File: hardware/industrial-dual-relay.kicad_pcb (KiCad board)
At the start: 2 copper layers, 40 x 40 mm, 34 parts, among them P1 CON-SENSOR2, P2 BOOT, P3 CONN_8, P4 Debug, Q2 G5Q-1, Q3 G5Q-1, U1 XMC1100, U4 DRILL, U5 DRILL, U6 DRILL, U7 DRILL

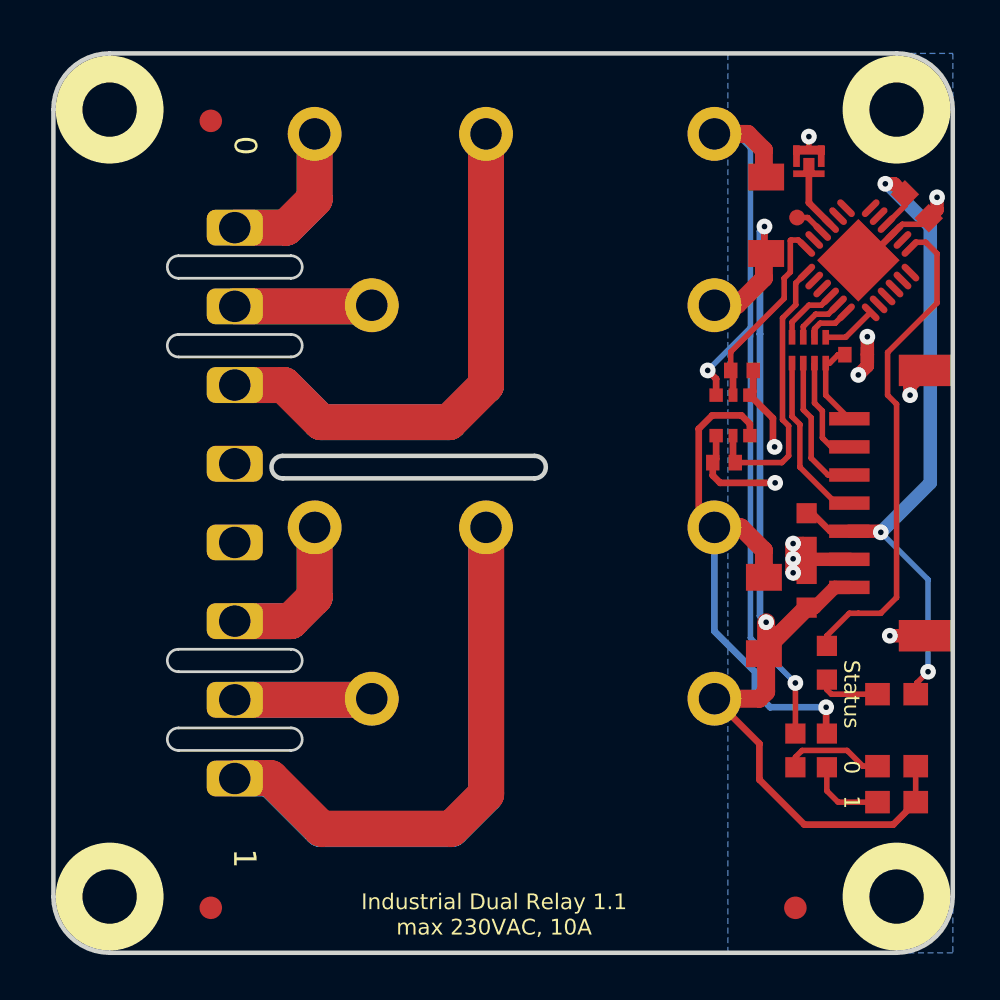
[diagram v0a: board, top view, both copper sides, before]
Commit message: Version 1.2: Updated relay footprint
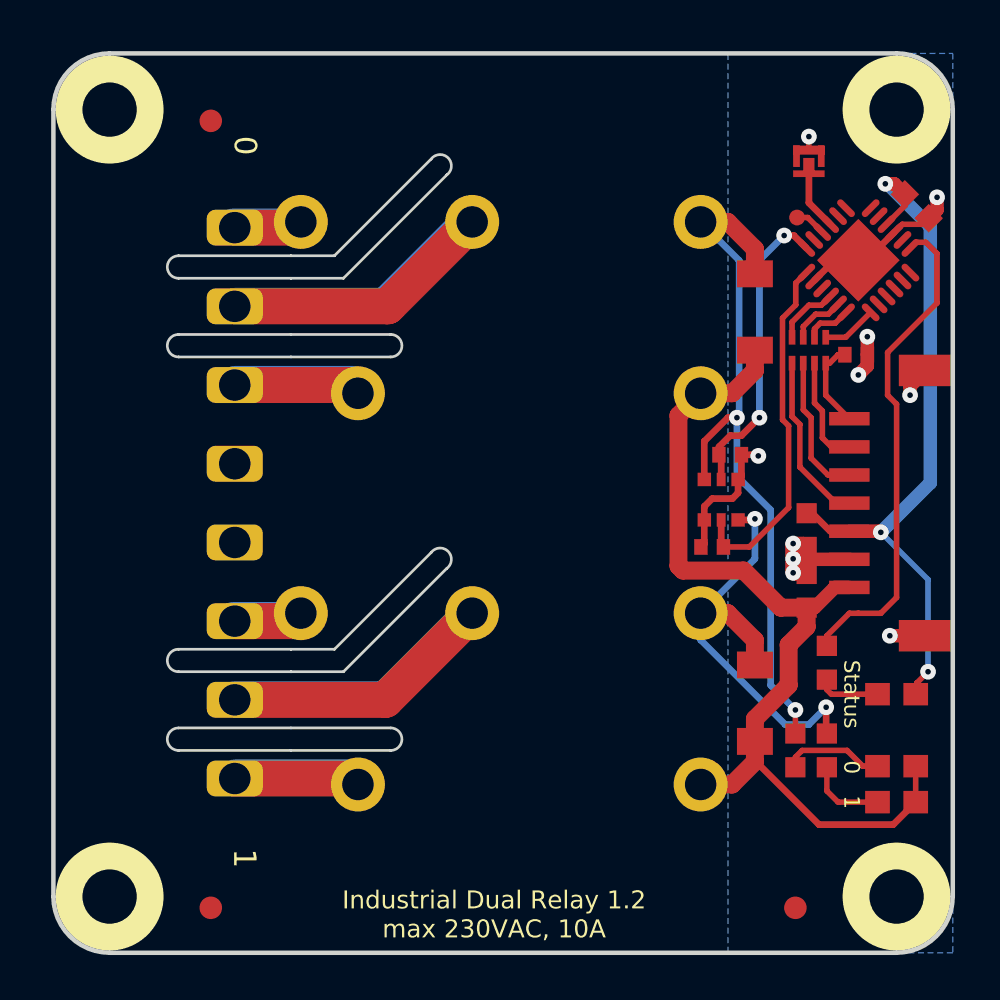
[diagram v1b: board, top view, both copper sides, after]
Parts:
- moved VAL 6.26 mm to (156.5, 104.2)
- moved D4 4.33 mm to (163.3, 95.7)
- moved VAL 4.10 mm to (156.5, 95.7)
- moved Q2 3.96 mm to (160.9, 99.3)
- moved D5 3.92 mm to (163.3, 113.1)
- moved Q3 3.86 mm to (160.9, 116.7)
- moved R4 3.79 mm to (161.4, 106.1)
- moved R5 3.79 mm to (162.2, 102.0)
- moved locked 3.79 mm to (161.8, 104.0)
- moved G*** 2.80 mm to (156.5, 113.8)
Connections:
- U1 pad 11: (no net) -> unconnected-(U1-Pad11)
- U1 pad 12: (no net) -> unconnected-(U1-Pad12)
- U1 pad 13: (no net) -> unconnected-(U1-Pad13)
- U1 pad 14: (no net) -> unconnected-(U1-Pad14)
- U1 pad 17: (no net) -> unconnected-(U1-Pad17)
- U1 pad 2: (no net) -> unconnected-(U1-Pad2)
- U1 pad 20: (no net) -> GND
- U1 pad 21: (no net) -> unconnected-(U1-Pad21)
- U1 pad 3: (no net) -> unconnected-(U1-Pad3)
- U1 pad 4: (no net) -> unconnected-(U1-Pad4)
- U1 pad 5: (no net) -> unconnected-(U1-Pad5)
- U1 pad 6: (no net) -> unconnected-(U1-Pad6)
- U1 pad 8: (no net) -> unconnected-(U1-Pad8)
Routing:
- net Net-(P3-Pad8): track 49.2 -> 10.8 mm
- net Net-(P3-Pad3): track 47.4 -> 10.8 mm
- net Net-(P3-Pad7): track 12.2 -> 24.3 mm
- net Net-(P3-Pad2): track 12.2 -> 24.3 mm
- net Net-(P3-Pad6): track 14.2 -> 5.67 mm
- net Net-(P3-Pad1): track 14.0 -> 5.63 mm
- net +5V: track 48.2 -> 42.4 mm, vias 2 -> 0
- net RELAY0: track 8.88 -> 13.6 mm, vias 0 -> 2
- net Net-(D5-Pad1): track 24.4 -> 19.9 mm, vias 1 -> 2
- net Net-(D4-Pad1): track 36.5 -> 32.2 mm
- net RELAY1: track 12.4 -> 15.9 mm
- net GND: track 33.1 -> 32.0 mm, vias 11 -> 10
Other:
- outline, holes or cut-outs redrawn
- board text added: "Industrial Dual Relay 1.2 max 230VAC, 10A"
- board text removed: "Industrial Dual Relay 1.1 max 230VAC, 10A"

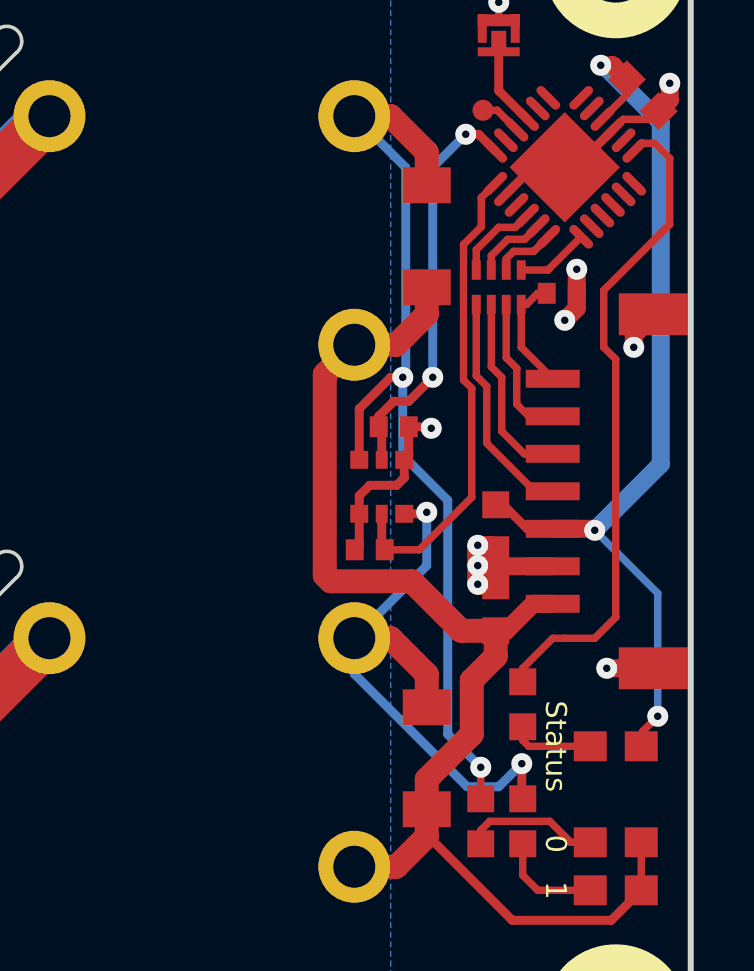
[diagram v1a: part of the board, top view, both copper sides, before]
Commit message: Version 1.2
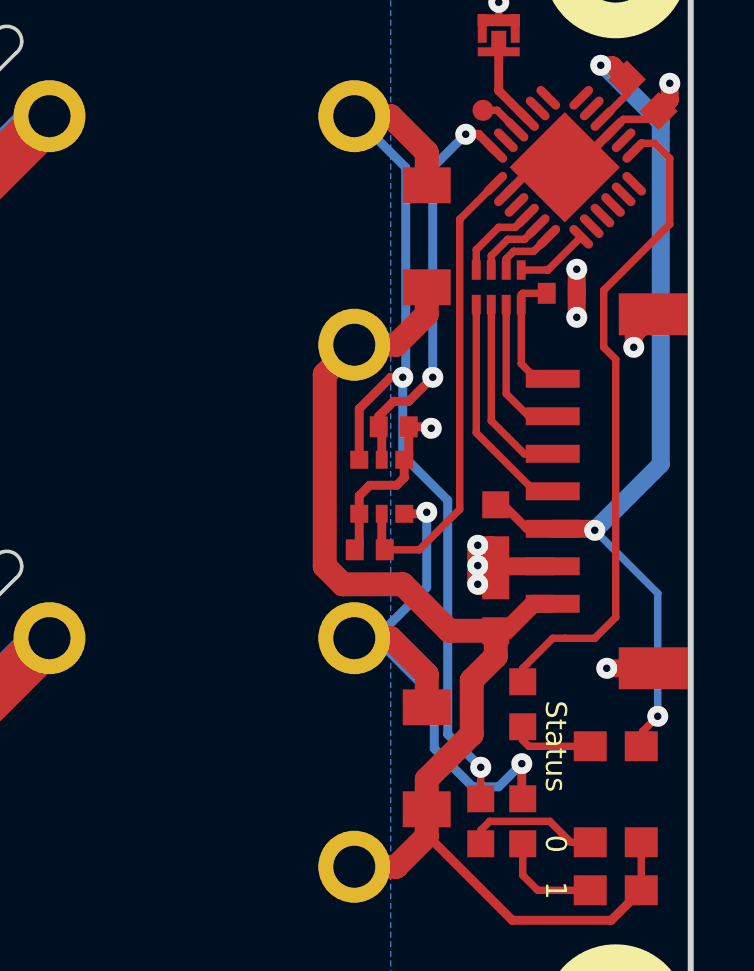
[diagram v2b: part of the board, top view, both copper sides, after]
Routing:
- net Net-(D5-Pad1): track 19.9 -> 20.7 mm
- net Net-(C2-Pad2): track 3.92 -> 4.43 mm

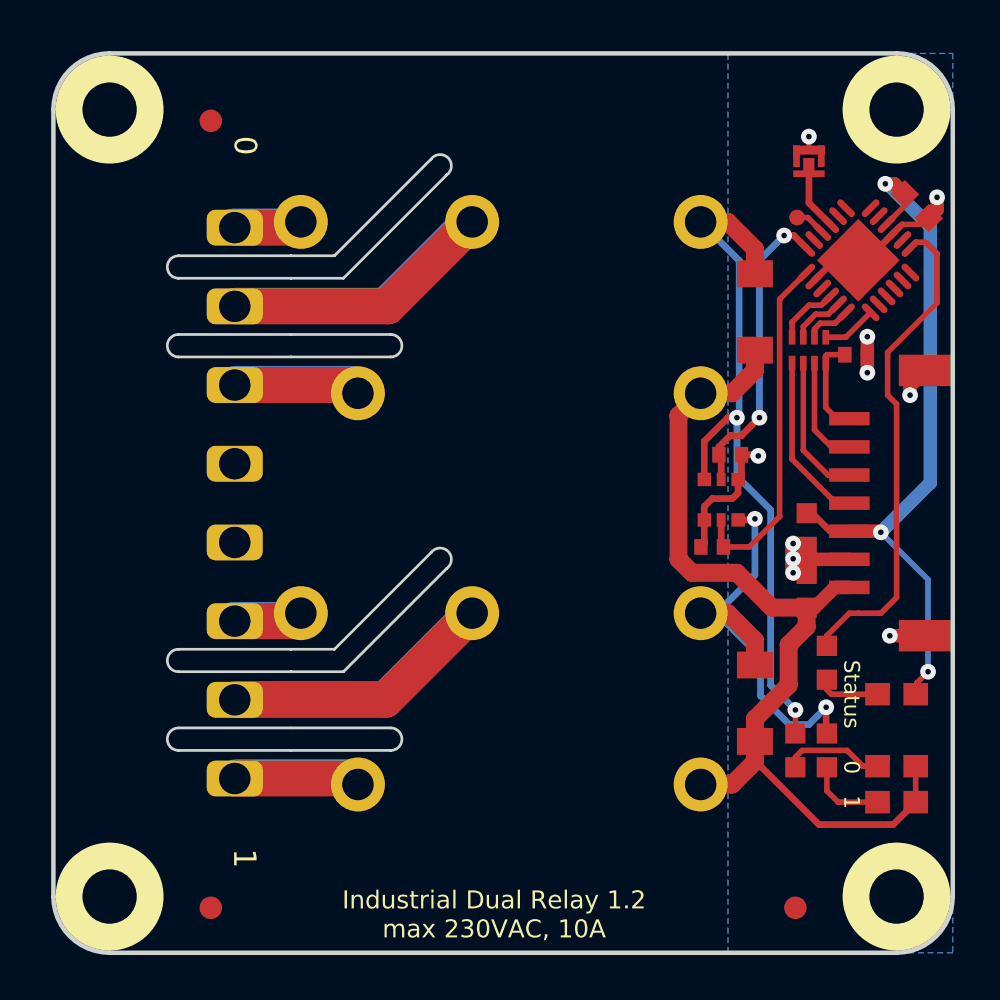
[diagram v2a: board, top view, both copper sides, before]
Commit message: Data cleanup.
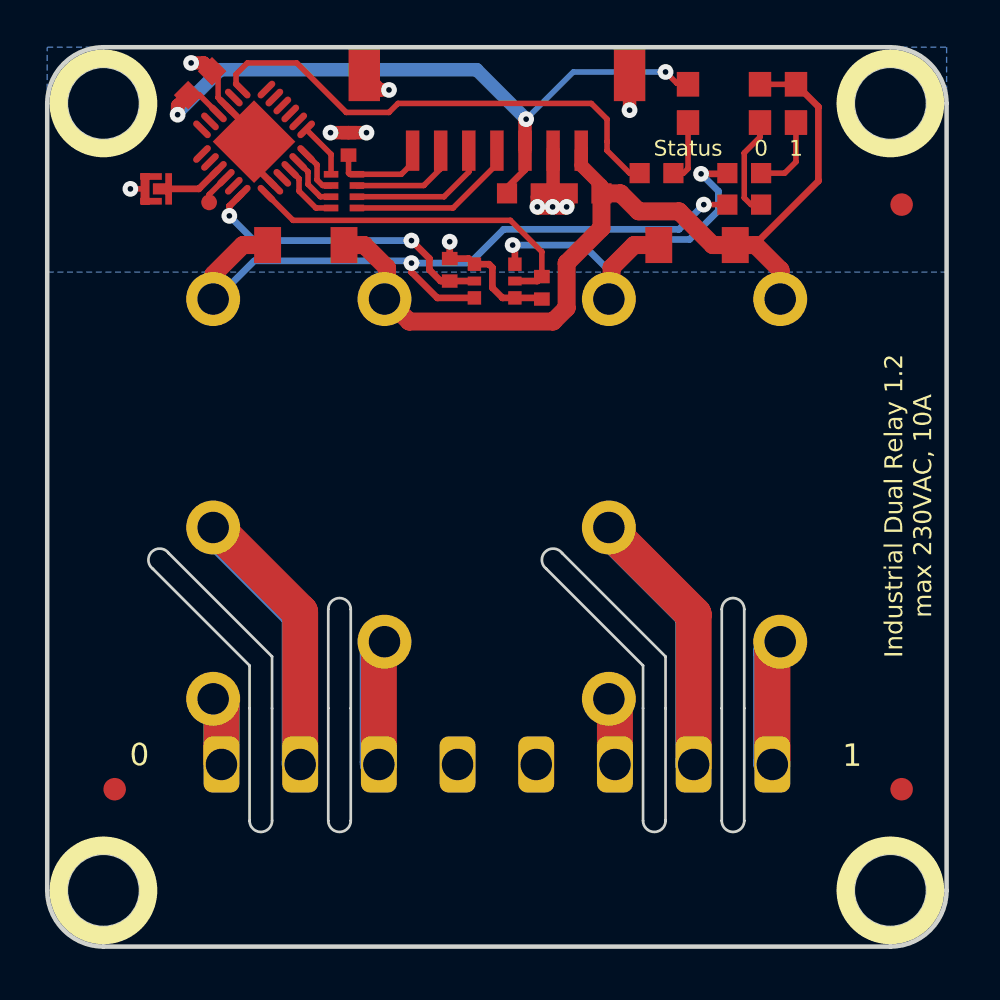
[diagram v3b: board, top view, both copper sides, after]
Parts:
- removed U7: DRILL, kicad-libraries:DRILL_NP
- added REF**: DRILL_NP_New, kicad-libraries:DRILL_NP_New, F.Cu at (134.3, 86.4)
- U4, U5, U6: footprint kicad-libraries:DRILL_NP -> kicad-libraries:DRILL_NP_New
- moved U4 35.3 mm to (169.3, 86.4), turned to 90 degrees
- moved U5 34.7 mm to (169.3, 121.4), turned to 90 degrees
- moved U6 34.7 mm to (134.3, 121.4), turned to 90 degrees
- moved C4 32.3 mm to (138.6, 85.5), turned to 45 degrees
- moved Fiducial_Mark 31.6 mm to (169.8, 90.9), turned to 90 degrees
- moved D3 31.4 mm to (165.1, 86.4), turned to -90 degrees
- moved Fiducial_Mark 31.2 mm to (169.8, 116.9), turned to 90 degrees
- moved D2 30.1 mm to (163.5, 86.4), turned to -90 degrees
- moved Fiducial_Mark 30.0 mm to (134.8, 116.9), turned to 90 degrees
- moved P2 29.1 mm to (136.7, 90.2), turned to 0 degrees
- moved P1 28.7 mm to (151.8, 83.9), turned to 180 degrees
- moved D1 27.9 mm to (160.3, 86.4), turned to -90 degrees
- moved U1 27.4 mm to (141.0, 88.1), turned to -135 degrees
- moved G*** 26.4 mm to (153.4, 85.5), turned to 180 degrees
- moved P4 26.2 mm to (139.0, 90.8), turned to 90 degrees
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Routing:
- net GND: track 31.8 -> 30.2 mm
- net Net-(D5-Pad1): track 20.7 -> 21.4 mm
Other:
- outline, holes or cut-outs redrawn
- board text added: "Copyright Tinkerforge GmbH 2023. This documentation describes Open Hardware and is licensed under the CERN OHL v. 1.1. You may redistribute and modify this documentation under the terms of the CERN OHL v.1.1. (http://ohwr.org/cernohl). This documentation is distributed WITHOUT ANY EXPRESS OR IMPLIED WARRANTY, INCLUDING OF MERCHANTABILITY, SATISFACTORY QUALITY AND FITNESS FOR A PARTICULAR PURPOSE.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"
- board text removed: "Copyright Tinkerforge GmbH 2017. This documentation describes Open Hardware and is licensed under the CERN OHL v. 1.1. You may redistribute and modify this documentation under the terms of the CERN OHL v.1.1. (http://ohwr.org/cernohl). This documentation is distributed WITHOUT ANY EXPRESS OR IMPLIED WARRANTY, INCLUDING OF MERCHANTABILITY, SATISFACTORY QUALITY AND FITNESS FOR A PARTICULAR PURPOSE.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"
